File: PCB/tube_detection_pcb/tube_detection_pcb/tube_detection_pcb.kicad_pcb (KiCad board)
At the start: 2 copper layers, 85 x 33 mm, 16 parts, among them J1 B6B-XH-A, U1 DM3CQF1003L01, U2 DM3CQF1003L01, U3 DM3CQF1003L01, U4 DM3CQF1003L01, U5 DM3CQF1003L01, U6 SN74HC165N

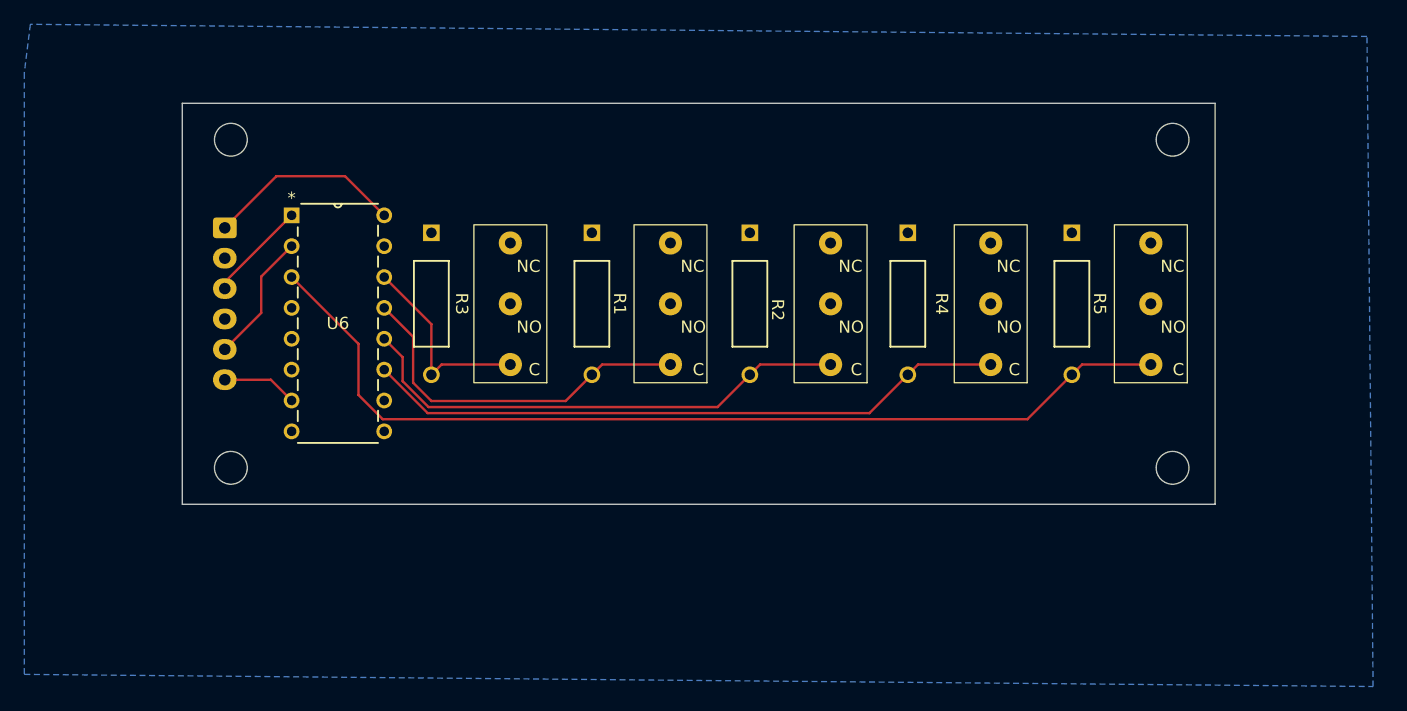
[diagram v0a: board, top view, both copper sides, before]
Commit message: PCB updates
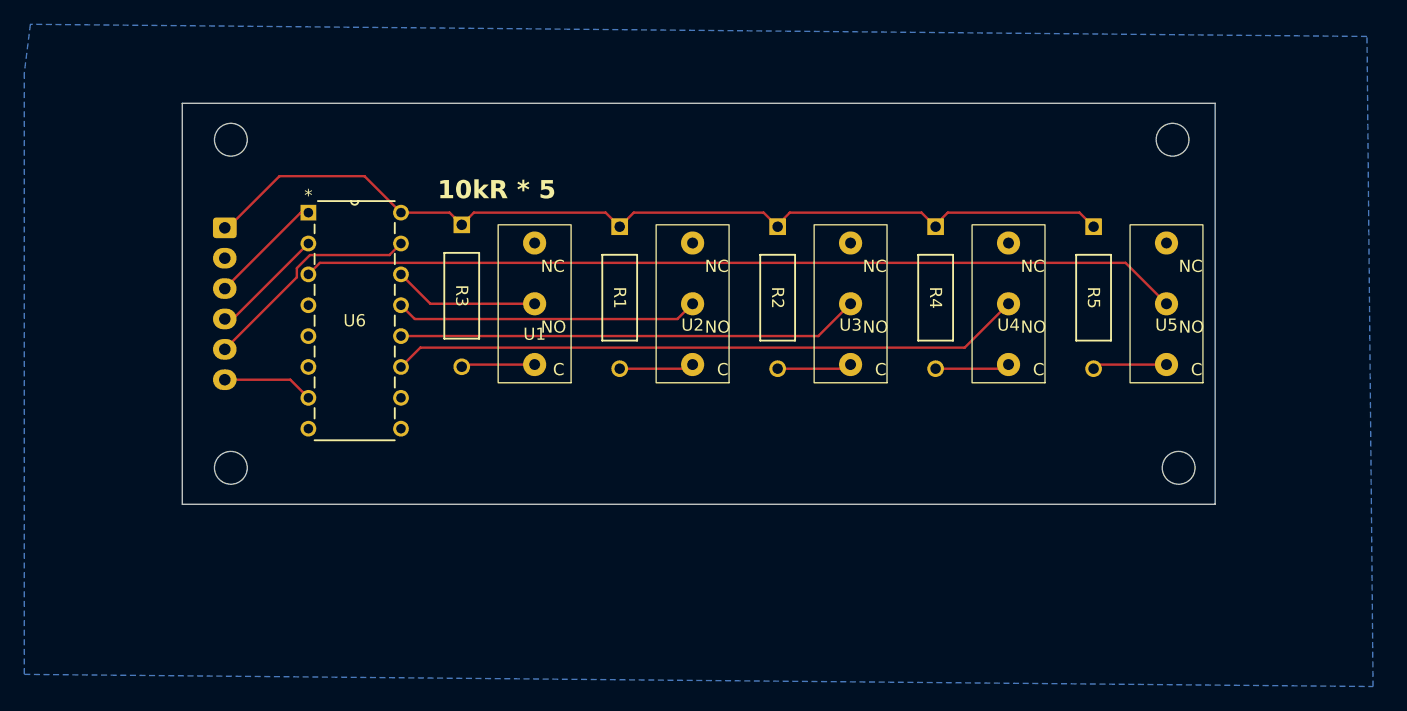
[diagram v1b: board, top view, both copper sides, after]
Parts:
- moved R3 2.59 mm to (123.0, 45.0)
- moved R1 2.34 mm to (136.0, 45.2)
- moved R2 2.34 mm to (149.0, 45.2)
- moved R4 2.34 mm to (162.0, 45.2)
- moved U1 2.00 mm to (129.0, 51.5)
- moved R5 1.86 mm to (175.0, 45.2)
- moved U2 1.82 mm to (142.0, 51.5)
- moved U3 1.64 mm to (155.0, 51.5)
- moved U4 1.47 mm to (168.0, 51.5)
- moved U6 1.40 mm to (118.0, 61.8)
- moved U5 1.29 mm to (181.0, 51.5)
- moved REF** 0.50 mm to (182.0, 65.0)
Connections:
- J1 pad 4: GND -> CLK
- J1 pad 5: CLK -> CSn
- U1 pad 2: GND -> Net-(U1-NO)
- U1 pad 3: unconnected-(U1-NC-Pad3) -> GND
- U2 pad 2: GND -> Net-(U2-NO)
- U2 pad 3: unconnected-(U2-NC-Pad3) -> GND
- U3 pad 2: GND -> Net-(U3-NO)
- U3 pad 3: unconnected-(U3-NC-Pad3) -> GND
- U4 pad 2: GND -> Net-(U4-NO)
- U4 pad 3: unconnected-(U4-NC-Pad3) -> GND
- U5 pad 2: GND -> Net-(U5-NO)
- U5 pad 3: unconnected-(U5-NC-Pad3) -> GND
- U6 pad 11: Net-(U4-C) -> Net-(U4-NO)
- U6 pad 12: Net-(U3-C) -> Net-(U3-NO)
- U6 pad 13: Net-(U2-C) -> Net-(U2-NO)
- U6 pad 14: Net-(U1-C) -> Net-(U1-NO)
- U6 pad 15: GND -> CSn
- U6 pad 3: Net-(U5-C) -> Net-(U5-NO)
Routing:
- net Net-(U5-C): track 79.9 -> 6.14 mm
- net Net-(U5-NO): track 0.00 -> 72.4 mm
- net +3V3: track 16.2 -> 78.9 mm
- net Net-(U4-NO): track 0.00 -> 52.2 mm
- net Net-(U4-C): track 53.1 -> 6.14 mm
- net Net-(U3-NO): track 0.00 -> 38.1 mm
- net Net-(U3-C): track 42.1 -> 6.14 mm
- net Net-(U2-NO): track 0.00 -> 25.0 mm
- net Net-(U2-C): track 30.2 -> 6.14 mm
- net CSn: track 0.00 -> 18.5 mm
- net Net-(U1-NO): track 0.00 -> 12.0 mm
- net Net-(U1-C): track 16.5 -> 6.08 mm
- net CLK: track 10.8 -> 9.45 mm
- net QH*: track 6.21 -> 7.50 mm
- net SH: track 8.31 -> 9.47 mm
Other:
- board text added: "10kR * 5"

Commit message: pcb finishing touches
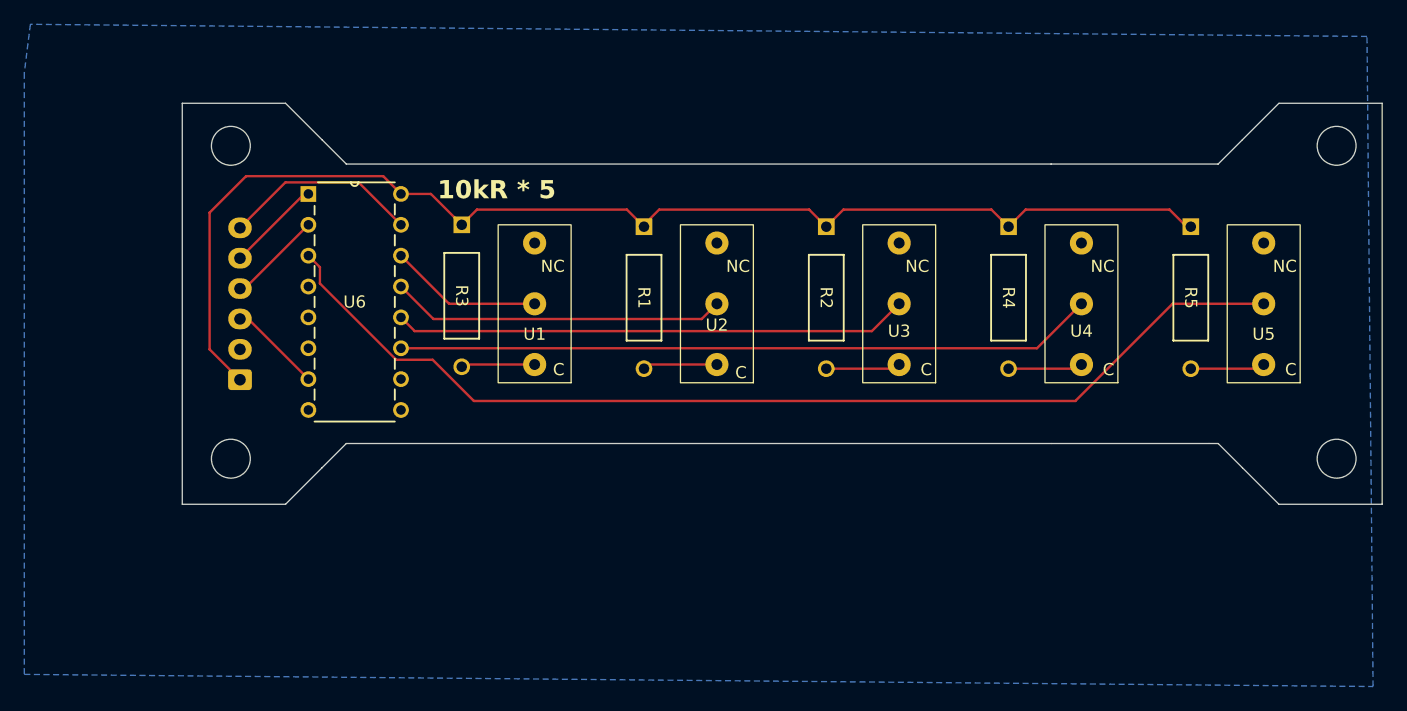
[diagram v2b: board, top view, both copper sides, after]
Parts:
- removed the REF** at (182.0, 65.0)
- removed the REF** at (181.5, 38.0)
- removed the REF** at (104.0, 65.0)
- removed the REF** at (104.0, 38.0)
- added REF**: MountingHole_3.2mm_M3, MountingHole:MountingHole_3.2mm_M3, F.Cu at (104.0, 64.2)
- added REF**: MountingHole_3.2mm_M3, MountingHole:MountingHole_3.2mm_M3, F.Cu at (195.0, 38.5)
- added REF**: MountingHole_3.2mm_M3, MountingHole:MountingHole_3.2mm_M3, F.Cu at (104.0, 38.5)
- added REF**: MountingHole_3.2mm_M3, MountingHole:MountingHole_3.2mm_M3, F.Cu at (195.0, 64.2)
- moved J1 12.6 mm to (104.8, 57.8), turned to 90 degrees
- moved R5 8.00 mm to (183.0, 45.2)
- moved U5 8.00 mm to (189.0, 51.5)
- moved R4 6.00 mm to (168.0, 45.2)
- moved U4 6.00 mm to (174.0, 51.5)
- moved R2 4.00 mm to (153.0, 45.2)
- moved U3 4.00 mm to (159.0, 51.5)
- moved R1 2.00 mm to (138.0, 45.2)
- moved U2 2.00 mm to (144.0, 51.5)
- moved U6 1.54 mm to (118.0, 60.2)
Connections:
- J1 pad 3: SH -> QH*
- J1 pad 5: CSn -> SH
- J1 pad 6: QH* -> CSn
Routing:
- net +3V3: track 78.9 -> 103.1 mm
- net Net-(U5-NO): track 72.4 -> 87.7 mm
- net Net-(U4-NO): track 52.2 -> 57.5 mm
- net Net-(U3-NO): track 38.1 -> 42.4 mm
- net Net-(U2-NO): track 25.0 -> 27.6 mm
- net CSn: track 18.5 -> 16.2 mm
- net SH: track 9.47 -> 7.82 mm
- net CLK: track 9.45 -> 7.80 mm
- net Net-(U1-NO): track 12.0 -> 12.6 mm
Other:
- board size 85 x 33 mm -> 98.8 x 33 mm
- board text removed: "NO"
